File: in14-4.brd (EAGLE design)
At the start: 132.1 x 41.9 mm, 15 parts, among them IC1 4094D, IC3 4094D, Q1 K155ID1, Q2 K155ID1, Q3 K155ID1, Q4 K155ID1

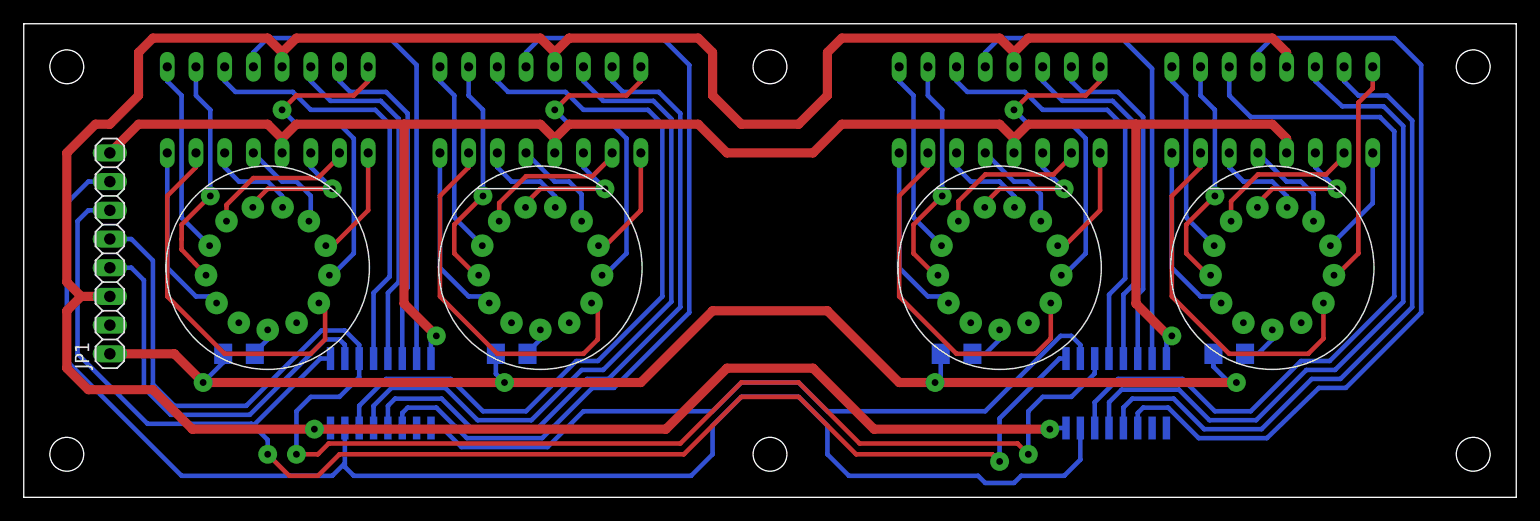
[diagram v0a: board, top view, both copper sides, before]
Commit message: Controller
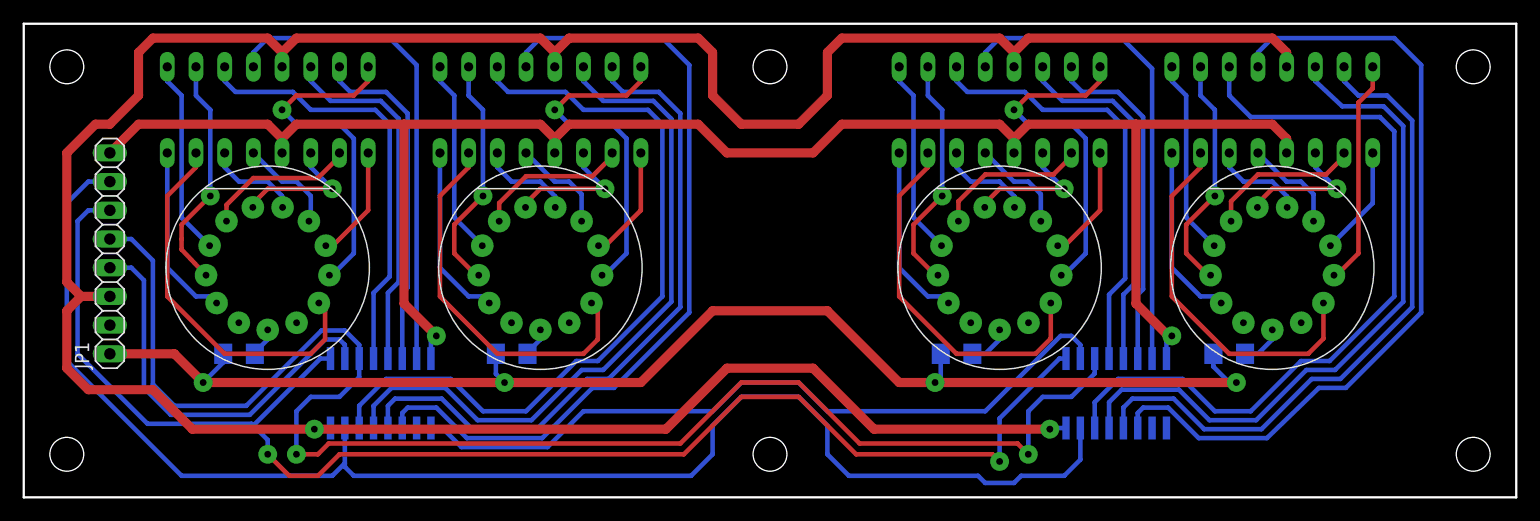
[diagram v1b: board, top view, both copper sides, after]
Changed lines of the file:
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@@
 <board>
 <plain>
-<wire x1="0" y1="0" x2="132.08" y2="0" width="0" layer="20"/>
-<wire x1="132.08" y1="0" x2="132.08" y2="41.91" width="0" layer="20"/>
-<wire x1="132.08" y1="41.91" x2="0" y2="41.91" width="0" layer="20"/>
-<wire x1="0" y1="41.91" x2="0" y2="0" width="0" layer="20"/>
+<wire x1="0" y1="0" x2="132.08" y2="0" width="0.2032" layer="20"/>
+<wire x1="132.08" y1="0" x2="132.08" y2="41.91" width="0.2032" layer="20"/>
+<wire x1="132.08" y1="41.91" x2="0" y2="41.91" width="0.2032" layer="20"/>
+<wire x1="0" y1="41.91" x2="0" y2="0" width="0.2032" layer="20"/>
 <hole x="3.81" y="38.1" drill="2.9972"/>
 <hole x="128.27" y="38.1" drill="2.9972"/>
